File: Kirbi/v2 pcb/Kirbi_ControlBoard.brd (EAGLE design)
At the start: 66 x 56 mm, 81 parts, among them U1 DEV-14057, U2 ICM-20948, U3 PCA9306, U4 RFM69HCW_SMT, U5 LM393ADR, U6 AP2114H-1.8TRG1, U7 AP2114H-3.3TRG1

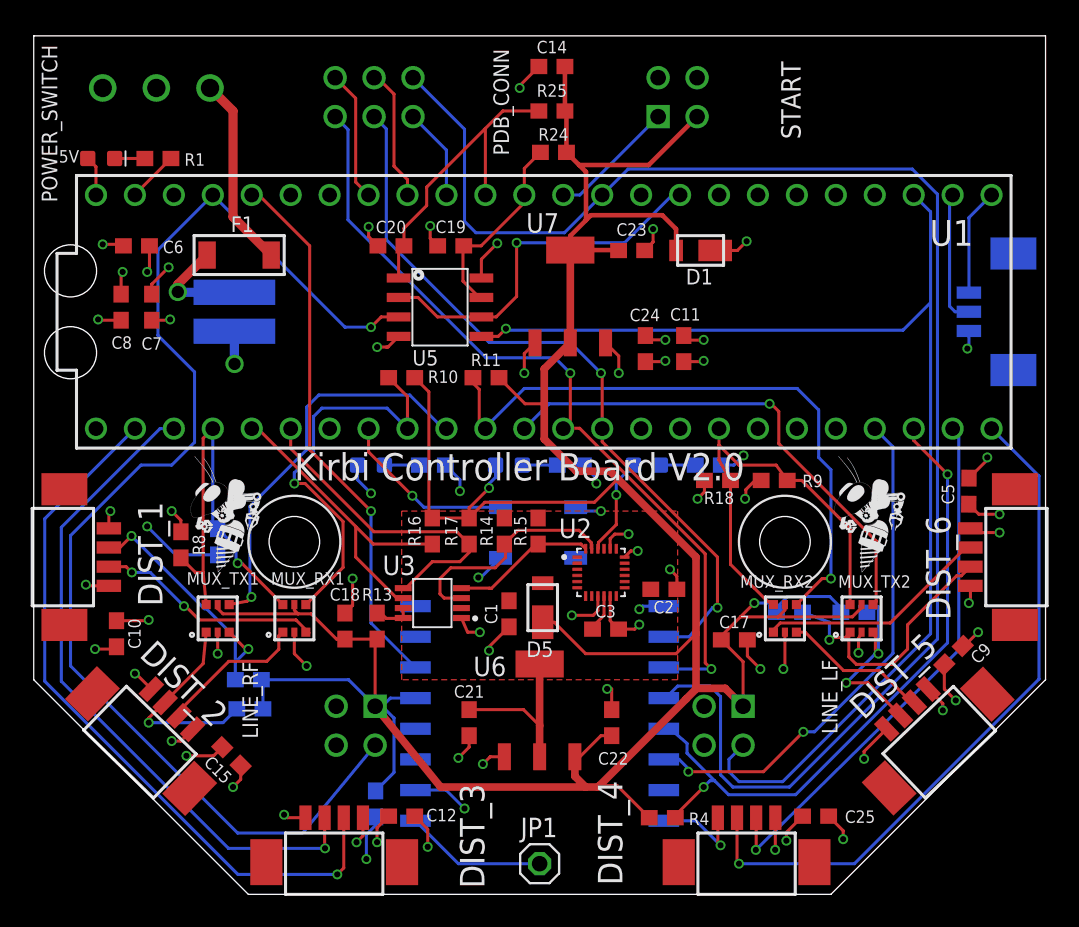
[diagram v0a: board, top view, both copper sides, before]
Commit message: Fixed doubled parts in Gucci and Kirbi Library
Fixed doubled parts in Gucci and Kirbi Library (IMU, Teensy)
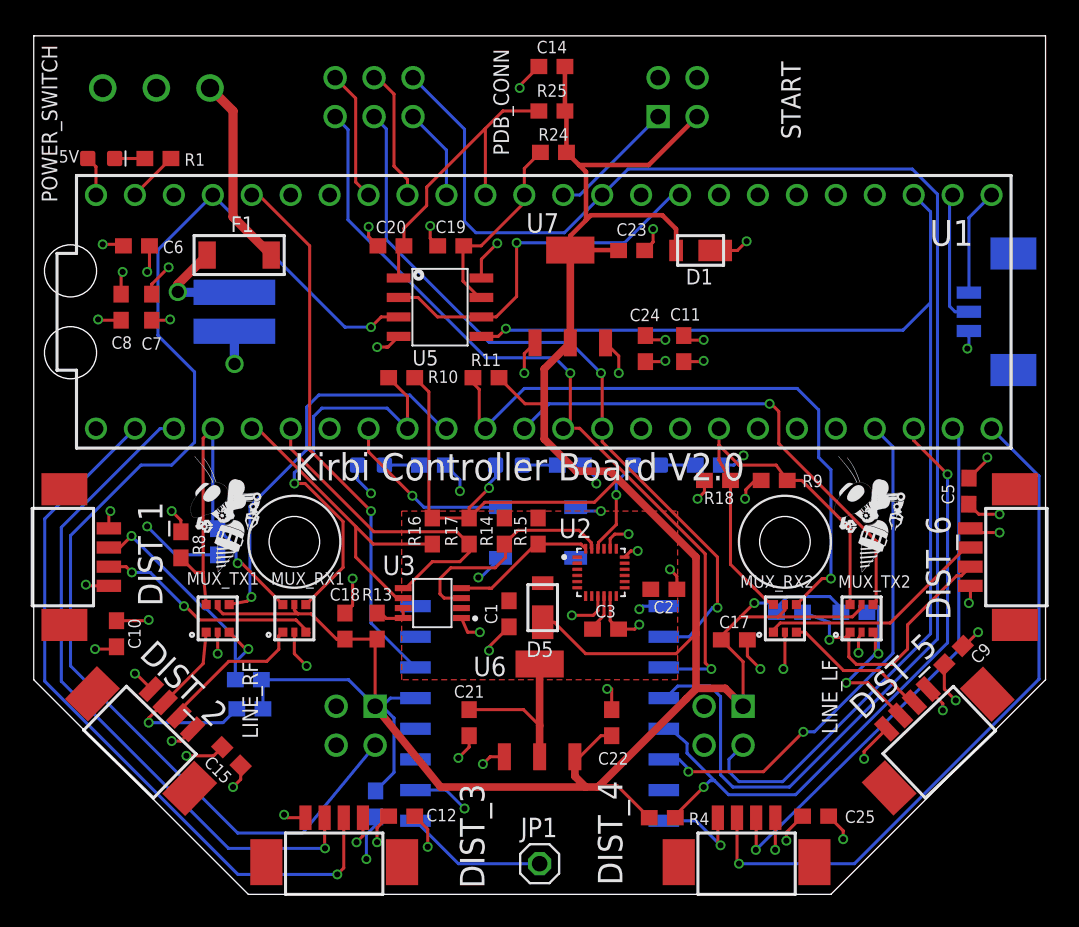
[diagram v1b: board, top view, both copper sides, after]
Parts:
- U1: value DEV-14057 -> TEENSY_3.6; device Kirbi_ControlBoard:TEENSY_3.6_DIL -> Gucci_ControlBoard:TEENSY_3.6
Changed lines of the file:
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@@
 </autorouter>
 <elements>
-<element name="U1" library="Kirbi_ControlBoard" package="TEENSY_3.6_DIL" value="DEV-14057" x="18" y="38" smashed="yes" rot="R90">
+<element name="U1" library="Gucci_ControlBoard" package="TEENSY_3.6" value="TEENSY_3.6" x="18" y="38" smashed="yes" rot="R90">
 <attribute name="DKPN" value="1568-1442-ND" x="18" y="38" size="1.778" layer="27" rot="R90" display="off"/>
 <attribute name="NAME" x="47.275" y="43.985" size="1.6764" layer="25" font="vector" rot="R180"/>
